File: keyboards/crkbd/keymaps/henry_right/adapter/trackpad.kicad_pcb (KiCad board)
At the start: 2 copper layers, 33.4 x 19.7 mm, 10 parts, among them J1 Conn_01x12, U1 Elite-C, U2 ProMicro, U3 NCP1117-3.3_SOT223, U4 TXB0104D

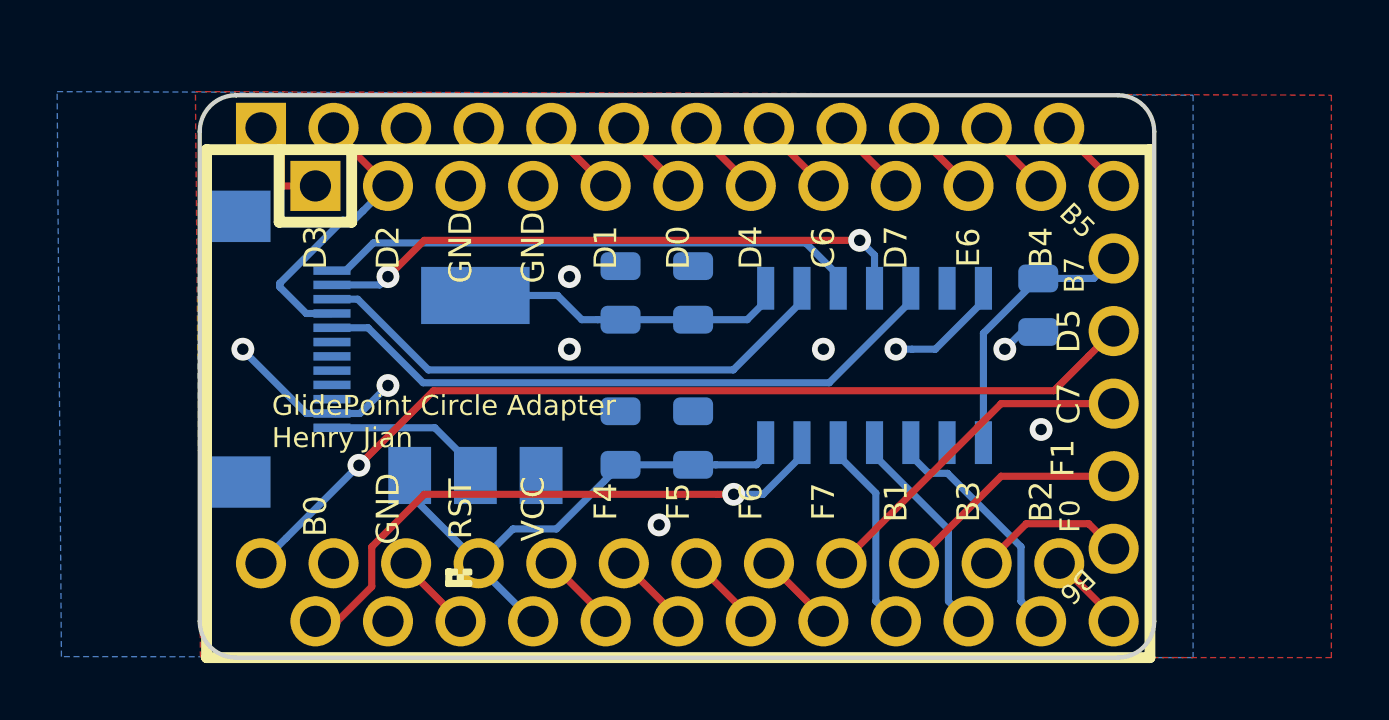
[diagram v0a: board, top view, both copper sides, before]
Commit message: 아트웍 시작 전.
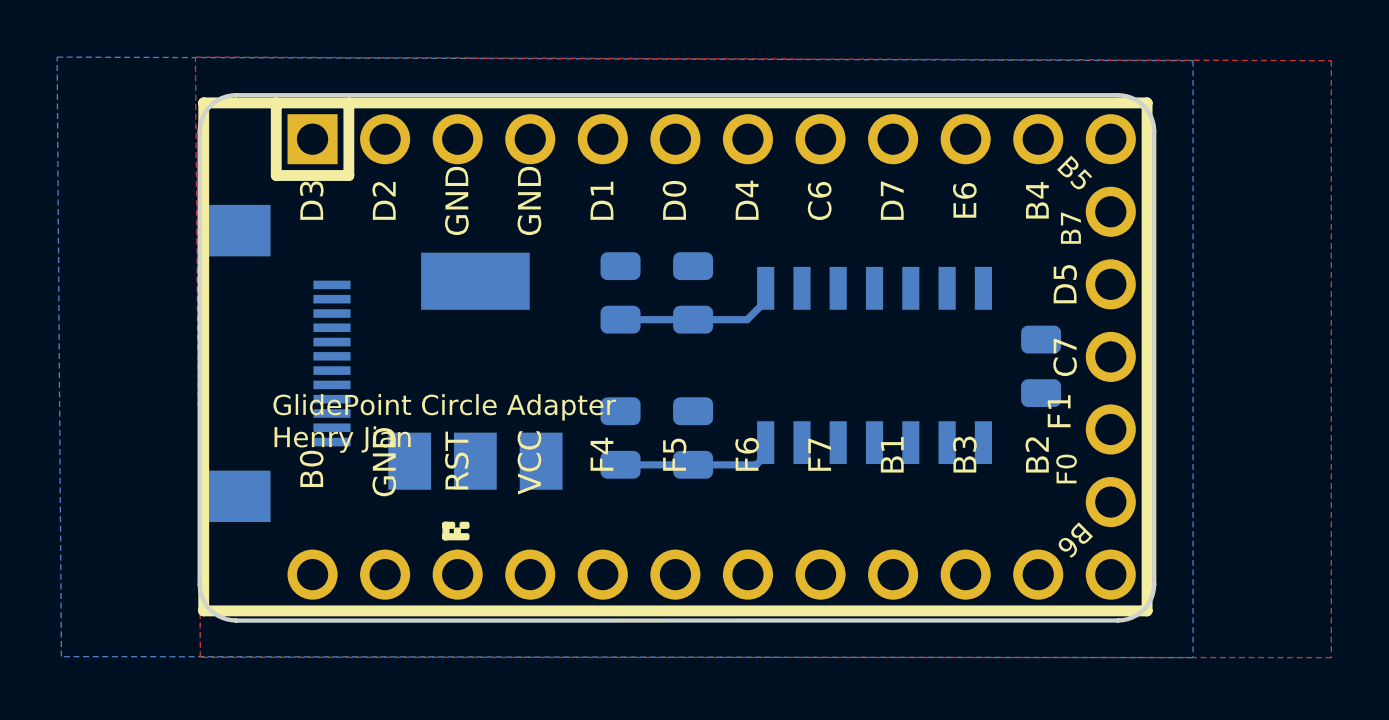
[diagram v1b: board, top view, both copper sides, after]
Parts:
- removed U2: ProMicro, trackpad:ArduinoProMicro-nf
- moved R1 2.14 mm to (127.0, 79.3), turned to 90 degrees
- moved U1 1.64 mm to (115.5, 79.0)
- moved J1 0.50 mm to (100.3, 79.2)
- moved U3 0.50 mm to (107.2, 79.5)
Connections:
- J1 pad 10: TP_CS_3V3 -> (no net)
- J1 pad 11: MISO_3V3 -> (no net)
- J1 pad 12: SCK_3V3 -> (no net)
- J1 pad 3: Net-(J1-Pad3) -> TP_SDA_3V3
- J1 pad 4: Net-(J1-Pad4) -> TP_SCL_3V3
- J1 pad 5: Net-(J1-Pad5) -> TP_BTN1_3V3
- J1 pad 6: Net-(J1-Pad6) -> (no net)
- J1 pad 7: Net-(J1-Pad7) -> (no net)
- J1 pad 8: MOSI_3V3 -> (no net)
- J1 pad 9: PD2 -> TP_DR_3V3
- U1 pad 1: PD3 -> (no net)
- U1 pad 10: PE6 -> (no net)
- U1 pad 11: PB4 -> (no net)
- U1 pad 12: PB5 -> (no net)
- U1 pad 13: PB6 -> (no net)
- U1 pad 14: MOSI -> (no net)
- U1 pad 15: MISO -> (no net)
- U1 pad 16: SCK -> (no net)
- U1 pad 17: PF7 -> (no net)
- U1 pad 18: PF6 -> (no net)
- U1 pad 19: PF5 -> (no net)
- U1 pad 2: PD2 -> (no net)
- U1 pad 20: PF4 -> (no net)
- U1 pad 22: RST -> (no net)
- U1 pad 24: TP_CS -> (no net)
- U1 pad 25: LVL_SHIFT -> TP_DR
- U1 pad 26: MAP_B0D5 -> (no net)
- U1 pad 27: MAP_B1C7 -> (no net)
- U1 pad 28: MAP_B3F1 -> (no net)
- U1 pad 29: MAP_B2F0 -> LVL_SHIFT
- U1 pad 7: PD4 -> (no net)
- U1 pad 8: PC6 -> (no net)
- U1 pad 9: PD7 -> (no net)
- U4 pad 10: MOSI -> TP_DR
- U4 pad 11: MISO -> (no net)
- U4 pad 12: SCK -> PD0
- U4 pad 13: TP_CS -> PD1
- U4 pad 2: TP_CS_3V3 -> TP_SDA_3V3
- U4 pad 3: SCK_3V3 -> TP_SCL_3V3
- U4 pad 4: MISO_3V3 -> TP_BTN1_3V3
- U4 pad 5: MOSI_3V3 -> TP_DR_3V3
- U4 pad 6: Net-(U4-Pad6) -> (no net)
- U4 pad 9: Net-(U4-Pad9) -> (no net)
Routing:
- net MAP_B0D5: track 33.2 -> 0.00 mm, vias 1 -> 0
- net MOSI_3V3: track 22.7 -> 0.00 mm
- net TP_CS: track 21.8 -> 0.00 mm, vias 1 -> 0
- net MISO_3V3: track 21.4 -> 0.00 mm, vias 2 -> 0
- net SCK_3V3: track 19.0 -> 0.00 mm
- net TP_CS_3V3: track 18.9 -> 0.00 mm
- net GND: track 13.9 -> 0.52 mm, vias 9 -> 0
- net +5V: track 19.0 -> 5.67 mm
- net MAP_B1C7: track 11.8 -> 0.00 mm
- net +3V3: track 17.1 -> 6.05 mm
- net PD2: track 10.9 -> 0.00 mm
- net LVL_SHIFT: track 9.47 -> 0.00 mm
- net MOSI: track 9.33 -> 0.00 mm
- net MAP_B3F1: track 8.25 -> 0.00 mm
- net SCK: track 7.89 -> 0.00 mm
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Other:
- board size 33.4 x 19.7 mm -> 33.4 x 18.4 mm
